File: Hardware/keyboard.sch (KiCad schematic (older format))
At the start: 139 parts

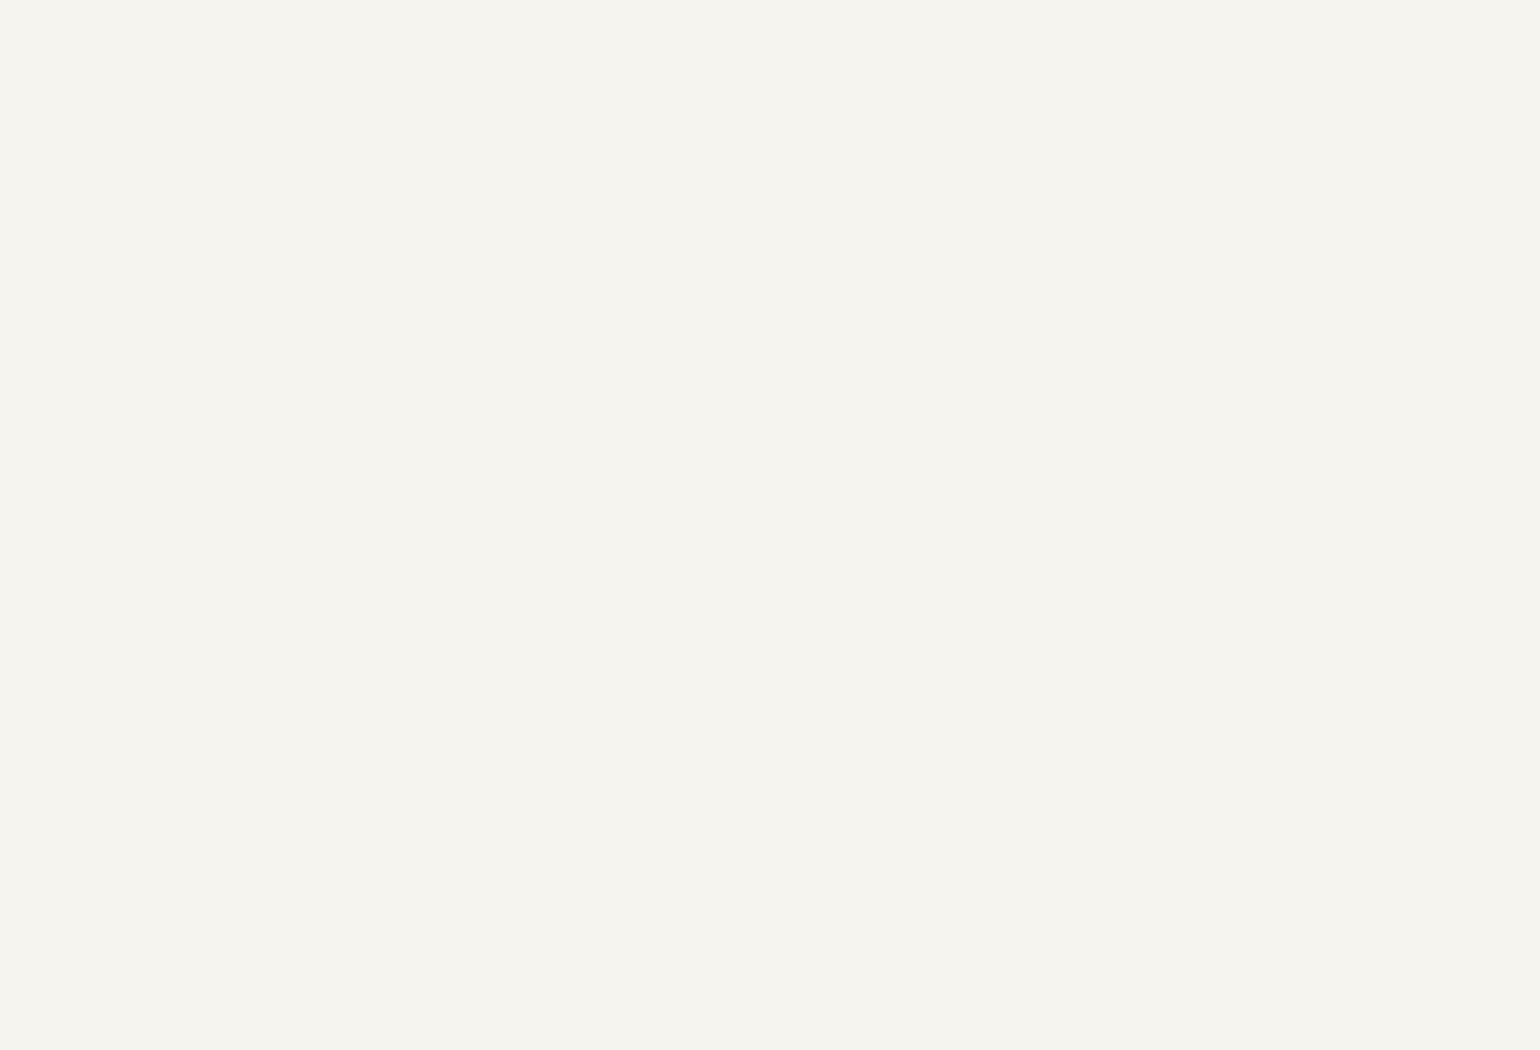
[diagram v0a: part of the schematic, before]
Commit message: Remove Tracks
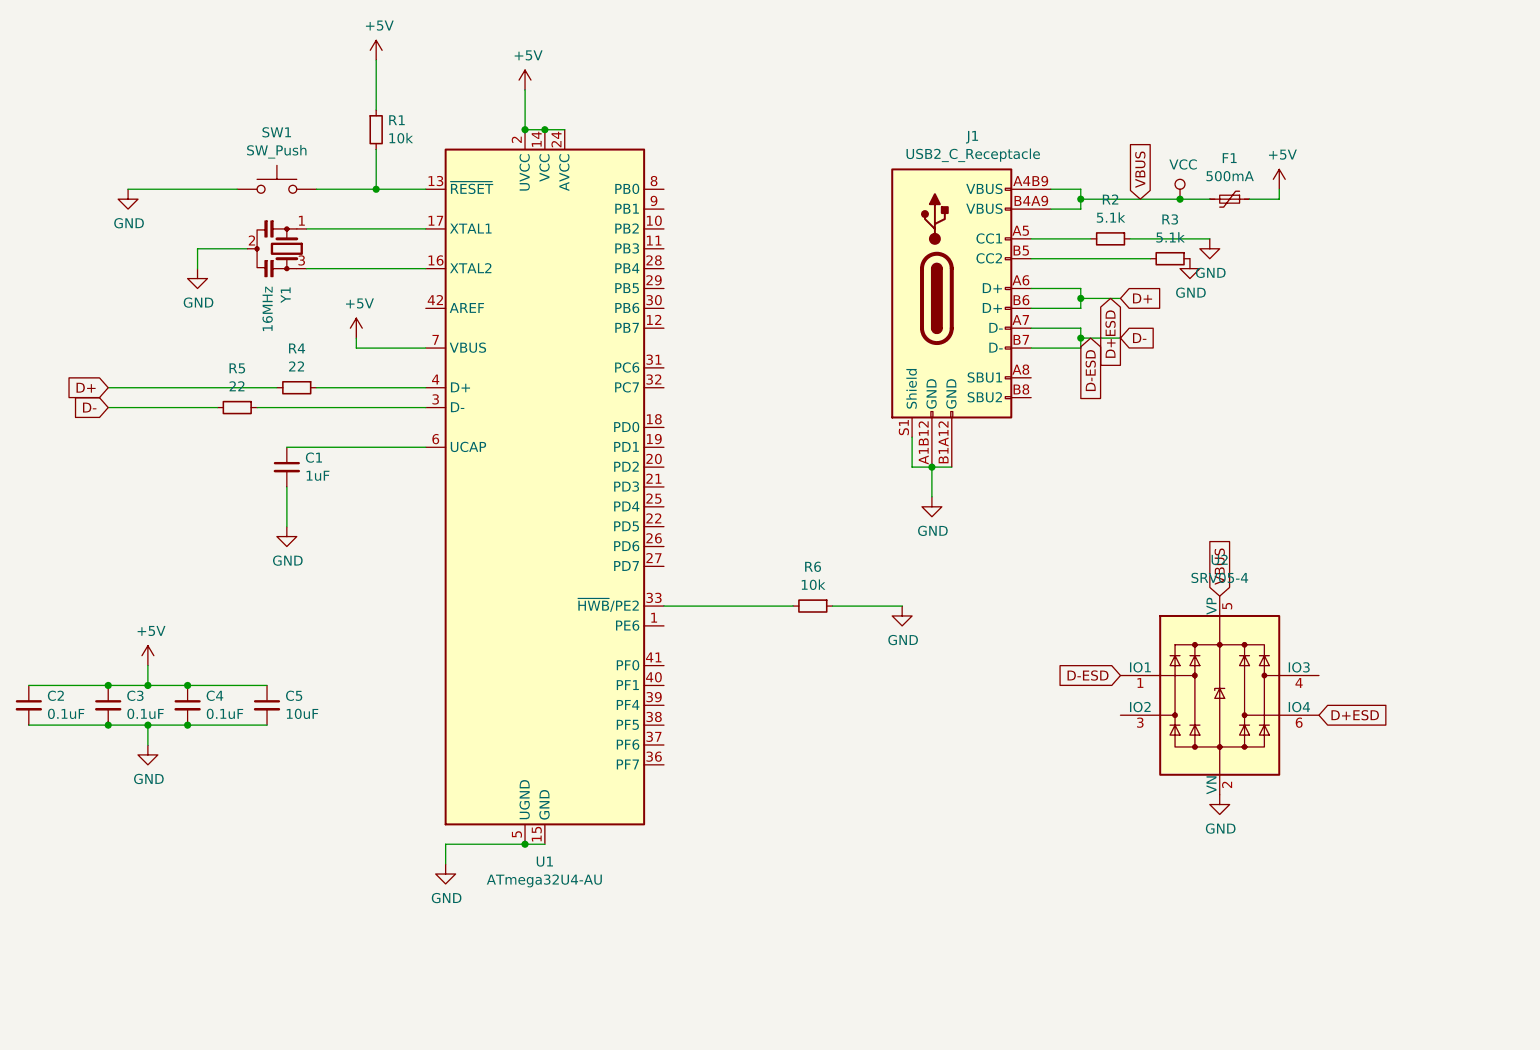
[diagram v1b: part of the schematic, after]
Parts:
- added C1: 1uF, Capacitor_SMD:C_0805_2012Metric, symbol Device:C_Small
- added C2, C3, C4: 0.1uF, Capacitor_SMD:C_0805_2012Metric, symbol Device:C_Small
- added C5: 10uF, Capacitor_SMD:C_0805_2012Metric, symbol Device:C_Small
- added F1: 500mA, Fuse:Fuse_1206_3216Metric, symbol Device:Polyfuse_Small
- added J1: USB2_C_Receptacle, usb-type-c:Mid_Mount-USB_C_HandSoldering, symbol usb-type-c:USB2_C_Receptacle
- added R1, R6: 10k, Resistor_SMD:R_0805_2012Metric, symbol Device:R_Small
- added R2, R3: 5.1k, Resistor_SMD:R_0805_2012Metric, symbol Device:R_Small
- added R4, R5: 22, Resistor_SMD:R_0805_2012Metric, symbol Device:R_Small
- added SW1: SW_Push, random-keyboard-parts:SKQG-1155865, symbol Switch:SW_Push
- added U1: ATmega32U4-AU, Package_QFP:TQFP-44_10x10mm_P0.8mm, symbol MCU_Microchip_ATmega:ATmega32U4-AU
- added U2: SRV05-4, Package_TO_SOT_SMD:SOT-23-6, symbol Power_Protection:SRV05-4
- added Y1: 16MHz, proj_local:Resonator_SMD_muRata_CSTxExxV-3Pin_3.0x1.1mm_HandSoldering_Compact, symbol Device:Resonator_Small
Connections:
- new net: R1.2, SW1.2, U1.13 (~RESET)
- new net: U1.16 (XTAL2), Y1.3
- new net: U1.17 (XTAL1), Y1.1
- new net: R5.1, U1.3 (D-)
- new net: R6.2, U1.33 (~HWB~/PE2)
- new net: R4.1, U1.4 (D+)
- new net: C1.1, U1.6 (UCAP)
- new net: J1.A5 (CC1), R2.2
- new net: J1.B5 (CC2), R3.2
- new net +5V: C2.1, C3.1, C4.1, C5.1, F1.1, R1.1, U1.14 (VCC), U1.2 (UVCC), U1.24 (AVCC), U1.34 (VCC), U1.44 (AVCC), U1.7 (VBUS)
- new net D+: J1.A6 (D+), J1.B6 (D+), R4.2, U2.6 (IO4)
- new net D-: J1.A7 (D-), J1.B7 (D-), R5.2, U2.1 (IO1)
- new net GND: C1.2, C2.2, C3.2, C4.2, C5.2, J1.A1B12 (GND), J1.B1A12 (GND), J1.S1 (Shield), R2.1, R3.1, R6.1, SW1.1, U1.15 (GND), U1.23 (GND), U1.35 (GND), U1.43 (GND), U1.5 (UGND), U2.2 (VN), Y1.2
- new net VCC: F1.2, J1.A4B9 (VBUS), J1.B4A9 (VBUS), U2.5 (VP)
